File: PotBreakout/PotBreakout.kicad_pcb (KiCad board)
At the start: 2 copper layers, 24.1 x 30.5 mm, 2 parts, among them J1 Conn_02x07_Odd_Even, U1 PDB183GTR21

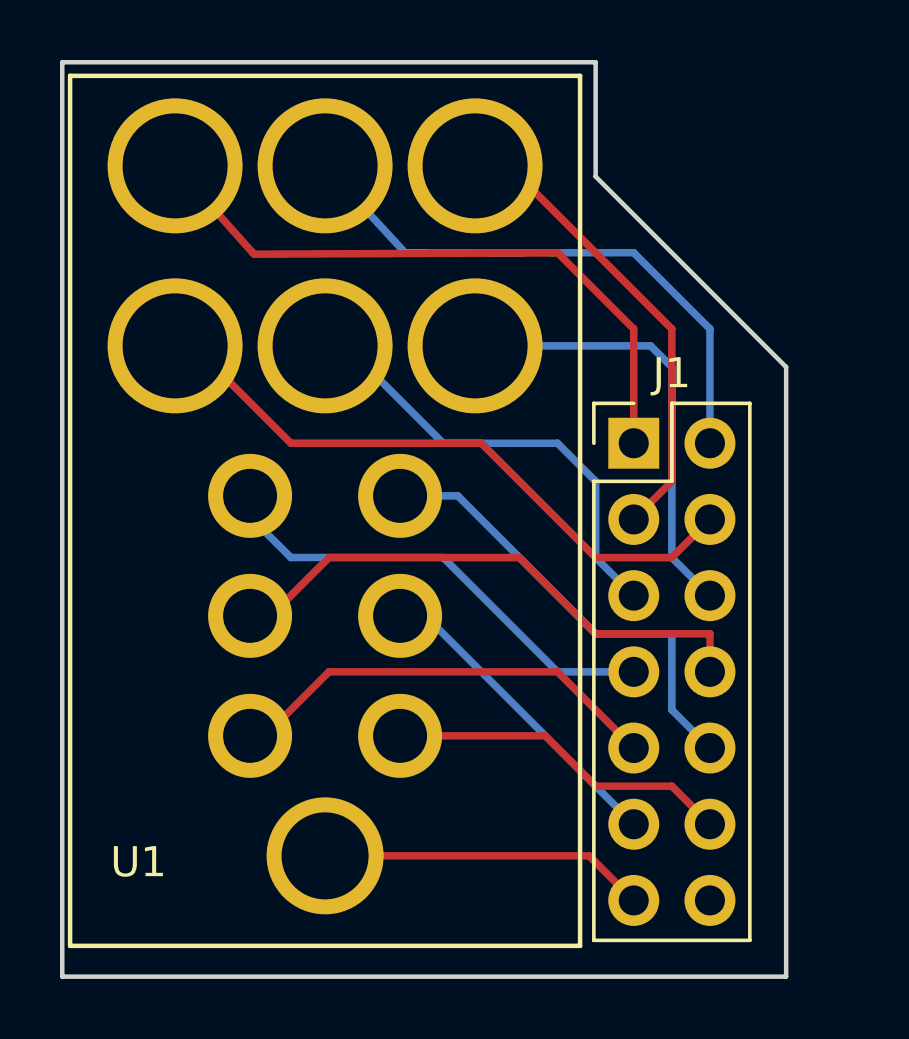
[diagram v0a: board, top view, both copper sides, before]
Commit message: Finalized pot breakout board
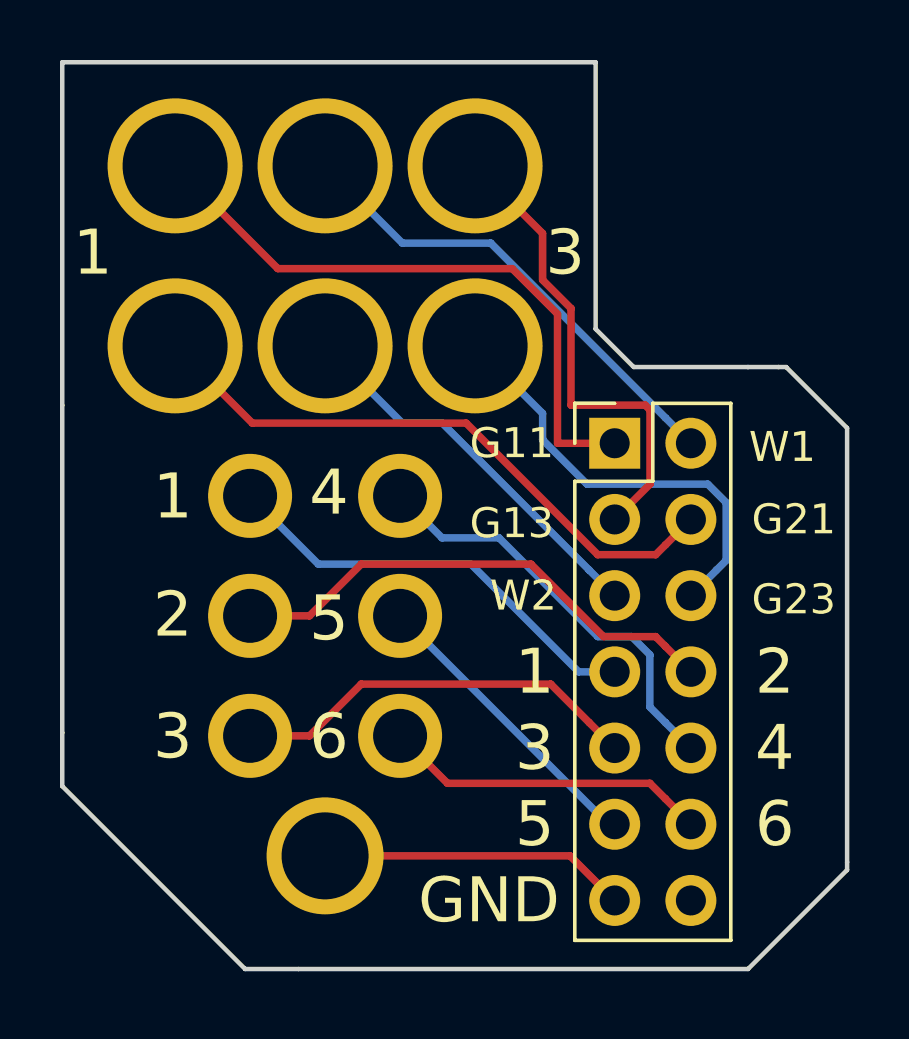
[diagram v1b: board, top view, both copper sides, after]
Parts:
- moved J1 0.63 mm to (160.7, 95.2)
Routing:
- net WIPE1: track 19.0 -> 16.0 mm
- net WIPE2: track 15.2 -> 13.1 mm
- net DPDT2: track 18.5 -> 16.9 mm
- net DPDT4: track 15.3 -> 14.2 mm
- net DPDT1: track 15.6 -> 14.6 mm
- net DPDT3: track 14.7 -> 13.8 mm
- net GANG21: track 21.3 -> 20.6 mm
- net DPDT6: track 11.5 -> 10.9 mm
- net GND: track 10.9 -> 10.3 mm
- net DPDT5: track 10.7 -> 10.0 mm
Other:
- board size 24.1 x 30.5 mm -> 26.2 x 30.2 mm
- board text added: "1"
- board text added: "2"
- board text added: "3"
- board text added: "4"
- board text added: "5"
- board text added: "6"
- board text added: "G11"
- board text added: "G13"
- board text added: "G21"
- board text added: "G23"
- board text added: "GND"
- board text added: "W1"
- board text added: "W2"
